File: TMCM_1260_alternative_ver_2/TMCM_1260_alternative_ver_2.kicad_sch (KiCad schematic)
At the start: 96 parts, among them J1 Motor, J2 CAN, J3 I/O, J4 Power, J8 Conn_02x06_Odd_Even, J9 Conn_02x06_Odd_Even, Q1 NVMFD5C650NLT1G, Q2 NVMFD5C650NLT1G, Q3 NVMFD5C650NLT1G, Q4 NVMFD5C650NLT1G, Q5 TLP185GR-TPL_SE, Q6 TLP185GR-TPL_SE, Q7 TLP185GR-TPL_SE, U1 LMZM23600V3SILR, U3 TCAN337, U4 TMC5160A-TA-T, U5 AS5047P-ATSM, U8 TMC4361A-LA-T

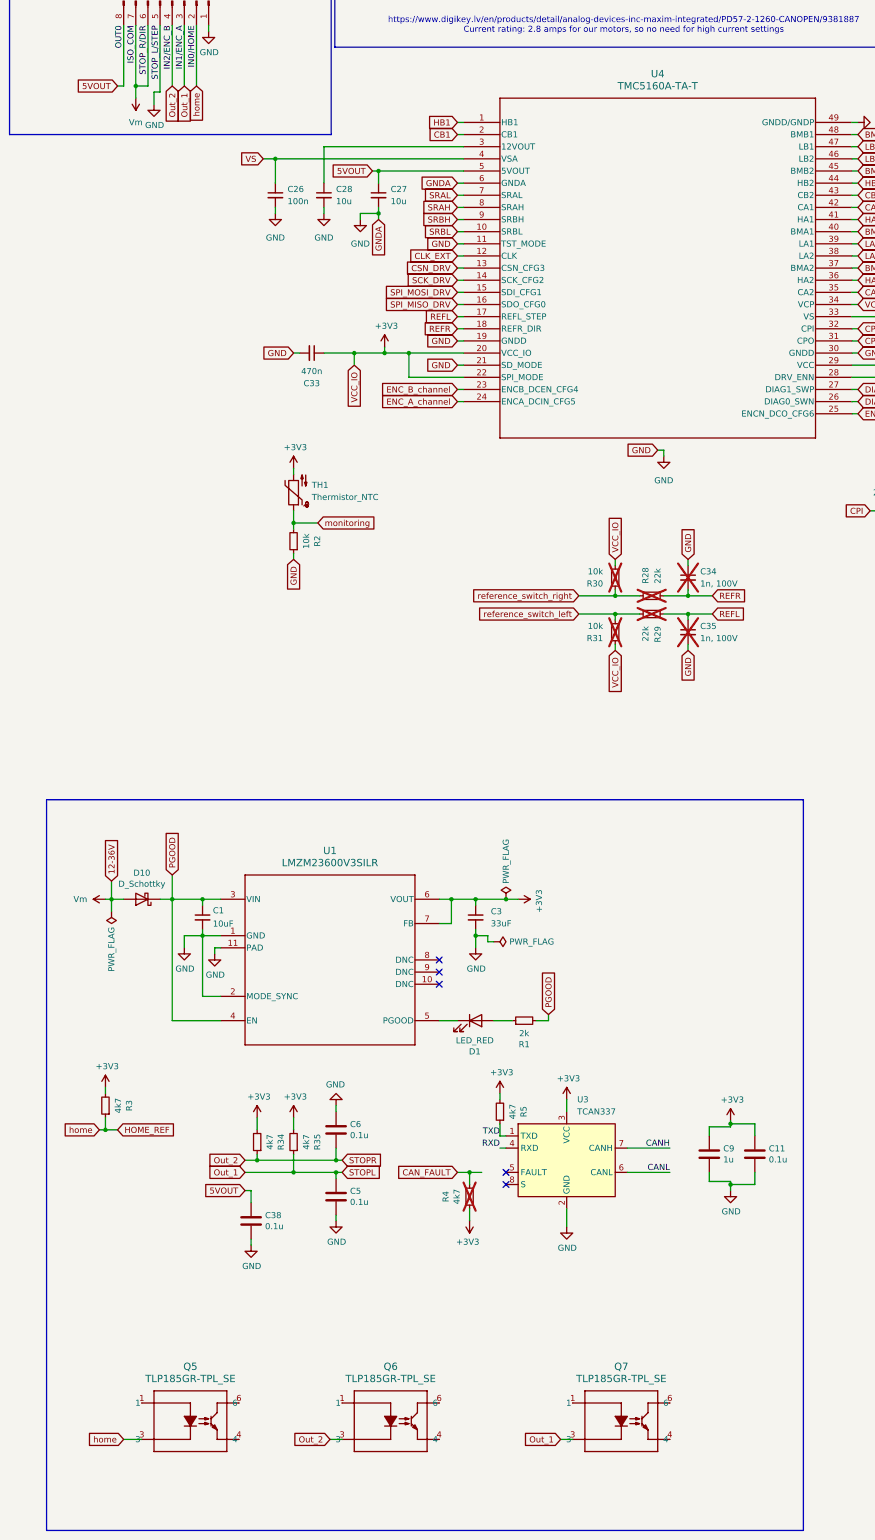
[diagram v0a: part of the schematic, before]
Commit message: finished
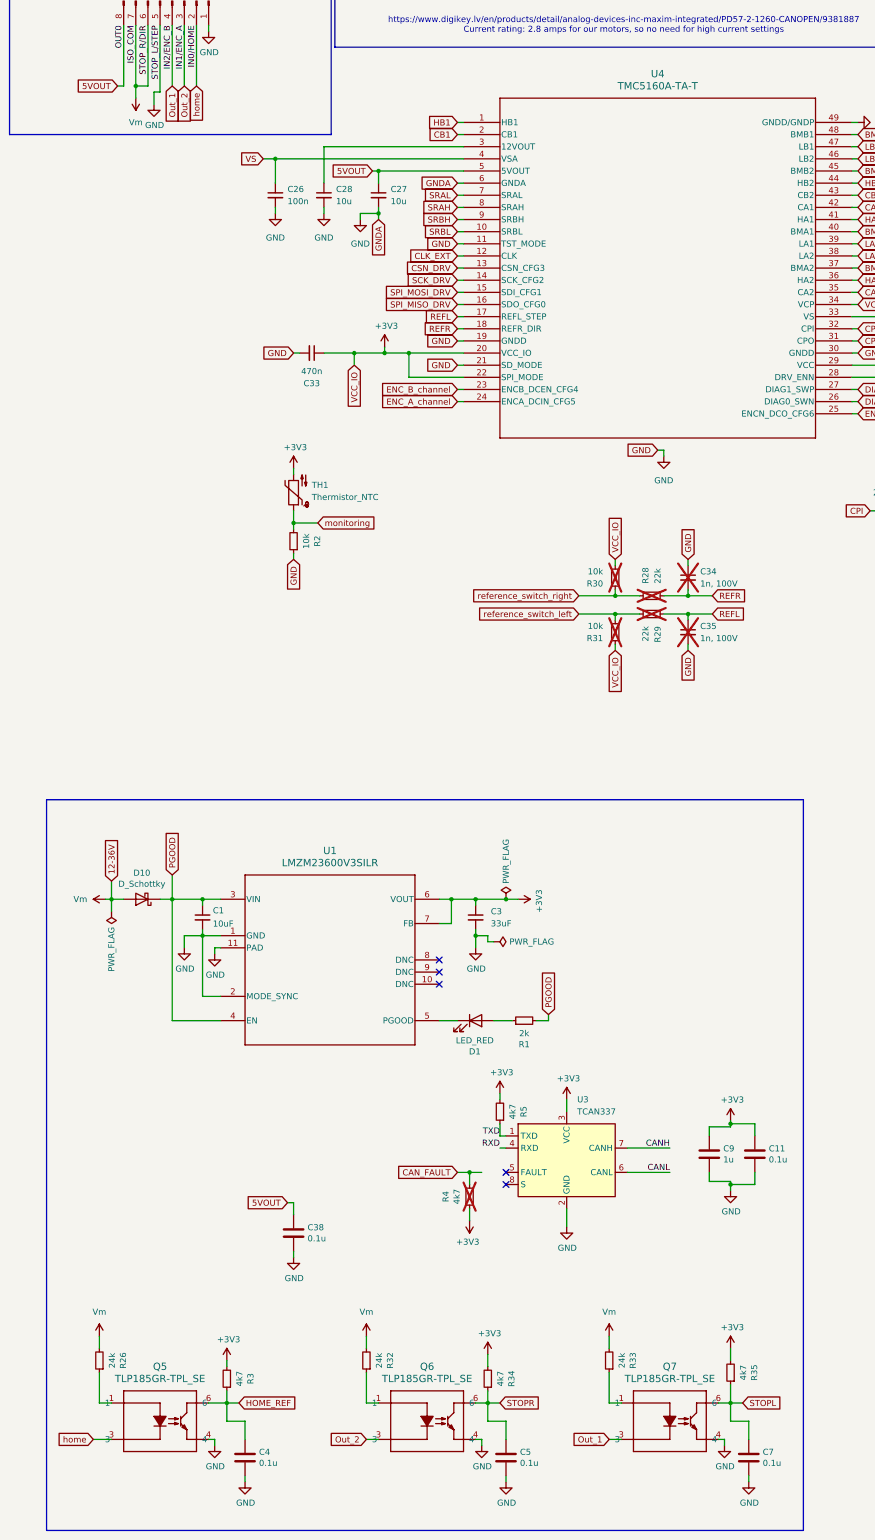
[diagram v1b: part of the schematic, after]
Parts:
- removed C6: 0.1u, Capacitor_SMD:C_0603_1608Metric, symbol Device:C
- added C4, C7: 0.1u, Capacitor_SMD:C_0402_1005Metric, symbol Device:C
- added R26, R32, R33: 24k, Resistor_SMD:R_0402_1005Metric, symbol Device:R_Small
- C5: footprint Capacitor_SMD:C_0603_1608Metric -> Capacitor_SMD:C_0402_1005Metric
- R3, R34, R35: footprint Resistor_SMD:R_0603_1608Metric_Pad0.98x0.95mm_HandSolder -> Resistor_SMD:R_0402_1005Metric
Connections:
- net GND: now also Q5.4, Q6.4, Q7.4, C4.2, C7.2
- net HOME_REF: now also Q5.6, C4.1; no longer J3.2 (Pin_2), Q5.3
- net Out_1: now also J3.4 (Pin_4); no longer C5.1, J3.3 (Pin_3), R35.1, U8.12 (STOPL)
- net Out_2: now also J3.3 (Pin_3); no longer J3.4 (Pin_4), R34.1, U8.14 (STOPR)
- net Vm: now also R26.2, R32.2, R33.2
- net at Q6.1: now also R32.1
- net STOPR: now reaches Q6.6
- net STOPR: now also C5.1, R34.1, U8.14 (STOPR)
- net at Q7.1: now also R33.1
- net STOPL: now reaches Q7.6
- net STOPL: now also R35.1, U8.12 (STOPL), C7.1
- net at Q5.1: now also R26.1
- new net home: J3.2 (Pin_2), Q5.3
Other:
- moved on the sheet: C38, Q5, Q6, Q7, R3
